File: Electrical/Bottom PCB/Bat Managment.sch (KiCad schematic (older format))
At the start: 15 parts, among them J301 Battery, SW301 SW_SPST, U301 MC78M05_TO252

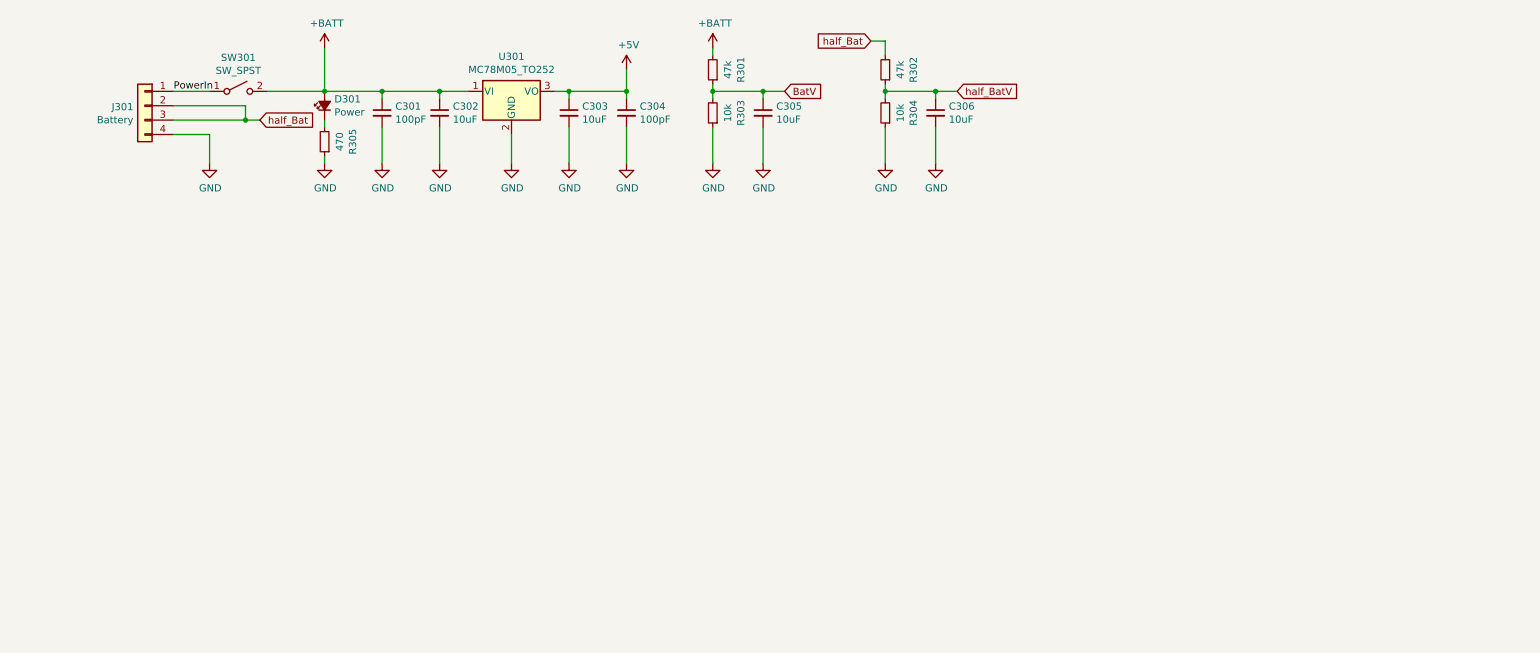
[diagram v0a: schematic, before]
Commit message: hello
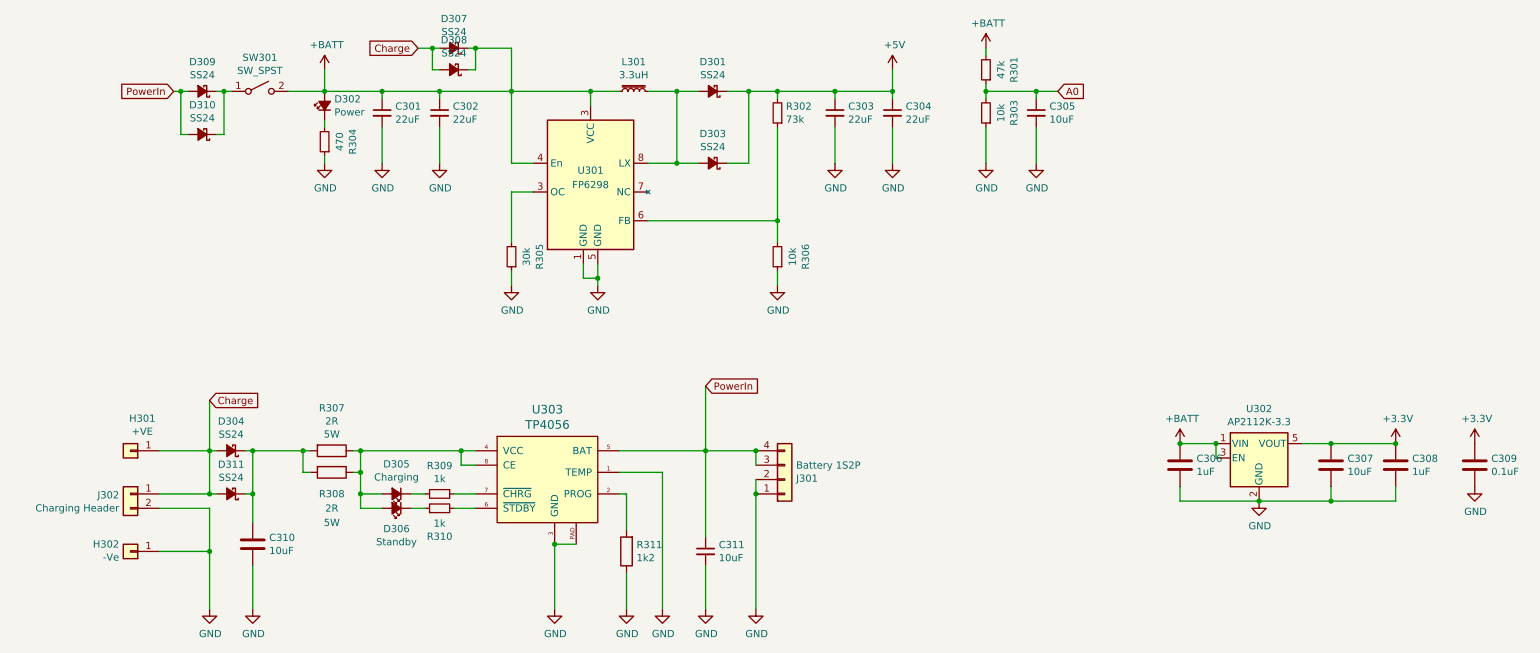
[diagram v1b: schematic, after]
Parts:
- removed C306: 10uF, Capacitor_SMD:C_0805_2012Metric_Pad1.15x1.40mm_HandSolder, symbol Device:C_Small
- removed R304: 10k, Resistor_SMD:R_0805_2012Metric_Pad1.15x1.40mm_HandSolder, symbol Device:R_Small
- removed U301: MC78M05_TO252, Package_TO_SOT_SMD:TO-252-2, symbol Regulator_Linear:MC78M05_TO252
- added C306, C308: 1uF, Capacitor_SMD:C_0603_1608Metric_Pad1.05x0.95mm_HandSolder, symbol Device:C
- added C307: 10uF, Capacitor_SMD:C_1206_3216Metric_Pad1.42x1.75mm_HandSolder, symbol Device:C
- added C309: 0.1uF, Capacitor_SMD:C_0603_1608Metric_Pad1.05x0.95mm_HandSolder, symbol Device:C
- added C310: 10uF, Capacitor_SMD:C_0805_2012Metric_Pad1.15x1.40mm_HandSolder, symbol Device:C
- added C311: 10uF, Capacitor_SMD:C_0805_2012Metric_Pad1.15x1.40mm_HandSolder, symbol Device:C_Small
- added D301, D303, D304, D307, D308, D309, D310, D311: SS24, Diode_SMD:D_SMB-SMC_Universal_Handsoldering, symbol Device:D_Schottky_Small_ALT
- added D305: Charging, LED_SMD:LED_0805_2012Metric_Pad1.15x1.40mm_HandSolder, symbol Device:LED_Small_ALT
- added D306: Standby, LED_SMD:LED_0805_2012Metric_Pad1.15x1.40mm_HandSolder, symbol Device:LED_Small_ALT
- added H301: +VE, TestPoint:TestPoint_Pad_D2.0mm, symbol Connector_Generic:Conn_01x01
- added H302: -Ve, TestPoint:TestPoint_Pad_D2.0mm, symbol Connector_Generic:Conn_01x01
- added J302: Charging Header, symbol Connector_Generic:Conn_01x02
- added L301: 3.3uH, symbol Device:L_Core_Iron_Small
- added R305: 30k, Resistor_SMD:R_0603_1608Metric_Pad0.98x0.95mm_HandSolder, symbol Device:R_Small
- added R306: 10k, Resistor_SMD:R_0603_1608Metric_Pad0.98x0.95mm_HandSolder, symbol Device:R_Small
- added R307, R308: 2R, Resistor_SMD:R_0603_1608Metric_Pad0.98x0.95mm_HandSolder, symbol Device:R
- added R309, R310: 1k, Resistor_SMD:R_0603_1608Metric_Pad0.98x0.95mm_HandSolder, symbol Device:R_Small
- added R311: 1k2, Resistor_SMD:R_0603_1608Metric_Pad0.98x0.95mm_HandSolder, symbol Device:R
- added U301: FP6298, Package_SO:SOIC-8_3.9x4.9mm_P1.27mm, symbol FP6298:FP6298
- added U302: AP2112K-3.3, Package_TO_SOT_SMD:SOT-23-5, symbol Regulator_Linear:AP2112K-3.3
- added U303: TP4056, Package_SO:SOP-8-1EP_4.57x4.57mm_P1.27mm_EP4.57x4.45mm_ThermalVias, symbol TP4056:TP4056
- C301, C304: value 100pF -> 22uF
- C302, C303: value 10uF -> 22uF
- J301: value Battery -> Battery 1S2P
- R301, R303: footprint Resistor_SMD:R_0805_2012Metric_Pad1.15x1.40mm_HandSolder -> Resistor_SMD:R_0603_1608Metric_Pad0.98x0.95mm_HandSolder
- R302: value 47k -> 73k; footprint Resistor_SMD:R_0805_2012Metric_Pad1.15x1.40mm_HandSolder -> Resistor_SMD:R_0603_1608Metric_Pad0.98x0.95mm_HandSolder
- R304: renamed from R305; footprint Resistor_SMD:R_0805_2012Metric_Pad1.15x1.40mm_HandSolder -> Resistor_SMD:R_0603_1608Metric_Pad0.98x0.95mm_HandSolder
- renumbered D301 to D302
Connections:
- net +5V: now also R302.2, D301.1 (K), D303.1 (K)
- net +BATT: now also C306.1, D307.1 (K), D308.1 (K), L301.1, U301.3 (VCC), U301.4 (En), U302.1 (VIN), U302.3 (EN)
- net GND: now also J301.1 (Pin_1), J301.2 (Pin_2), C306.2, C307.2, C308.2, C309.2, C310.2, C311.2, H302.1 (Pin_1), J302.2 (Pin_2), R305.1, R306.1, R311.1, U301.1 (GND), U301.5 (GND), U302.2 (GND), U303.1 (TEMP), U303.3 (GND), U303.PAD; no longer J301.4 (Pin_4)
- net PowerIn: now also J301.3 (Pin_3), J301.4 (Pin_4), C311.1, D309.2 (A), D310.2 (A), U303.5 (BAT); no longer J301.1 (Pin_1), SW301.1 (A)
- net BatV renamed A0
- removed net half_Bat: J301.2 (Pin_2), J301.3 (Pin_3), R302.2
- net half_BatV: no longer names the net of R302.1
- net half_BatV: now also R306.2, U301.6 (FB)
- new net: D309.1 (K), D310.1 (K), SW301.1 (A)
- new net: R305.2, U301.3 (VCC)
- new net: D301.2 (A), D303.2 (A), L301.2, U301.8 (LX)
- new net: D305.1 (K), R309.2
- new net: D305.2 (A), D306.2 (A), R307.1, R308.1, U303.4 (VCC), U303.8 (CE)
- new net: R309.1, U303.7 (~CHRG)
- new net: C310.1, D304.1 (K), D311.1 (K), R307.2, R308.2
- new net: R311.2, U303.2 (PROG)
- new net: R310.2, U303.6 (~STDBY)
- new net: D306.1 (K), R310.1
- new net +3V3: C307.1, C308.1, C309.1, U302.5 (VOUT)
- new net Charge: D304.2 (A), D307.2 (A), D308.2 (A), D311.2 (A), H301.1 (Pin_1), J302.1 (Pin_1)
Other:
- moved on the sheet: C303, C304, C305, J301, R301, R303, SW301
